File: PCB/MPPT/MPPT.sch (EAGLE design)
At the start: 2 parts, among them IC1 ACS711KEXLT-15AB-T, IC2 ACS711KEXLT-15AB-T

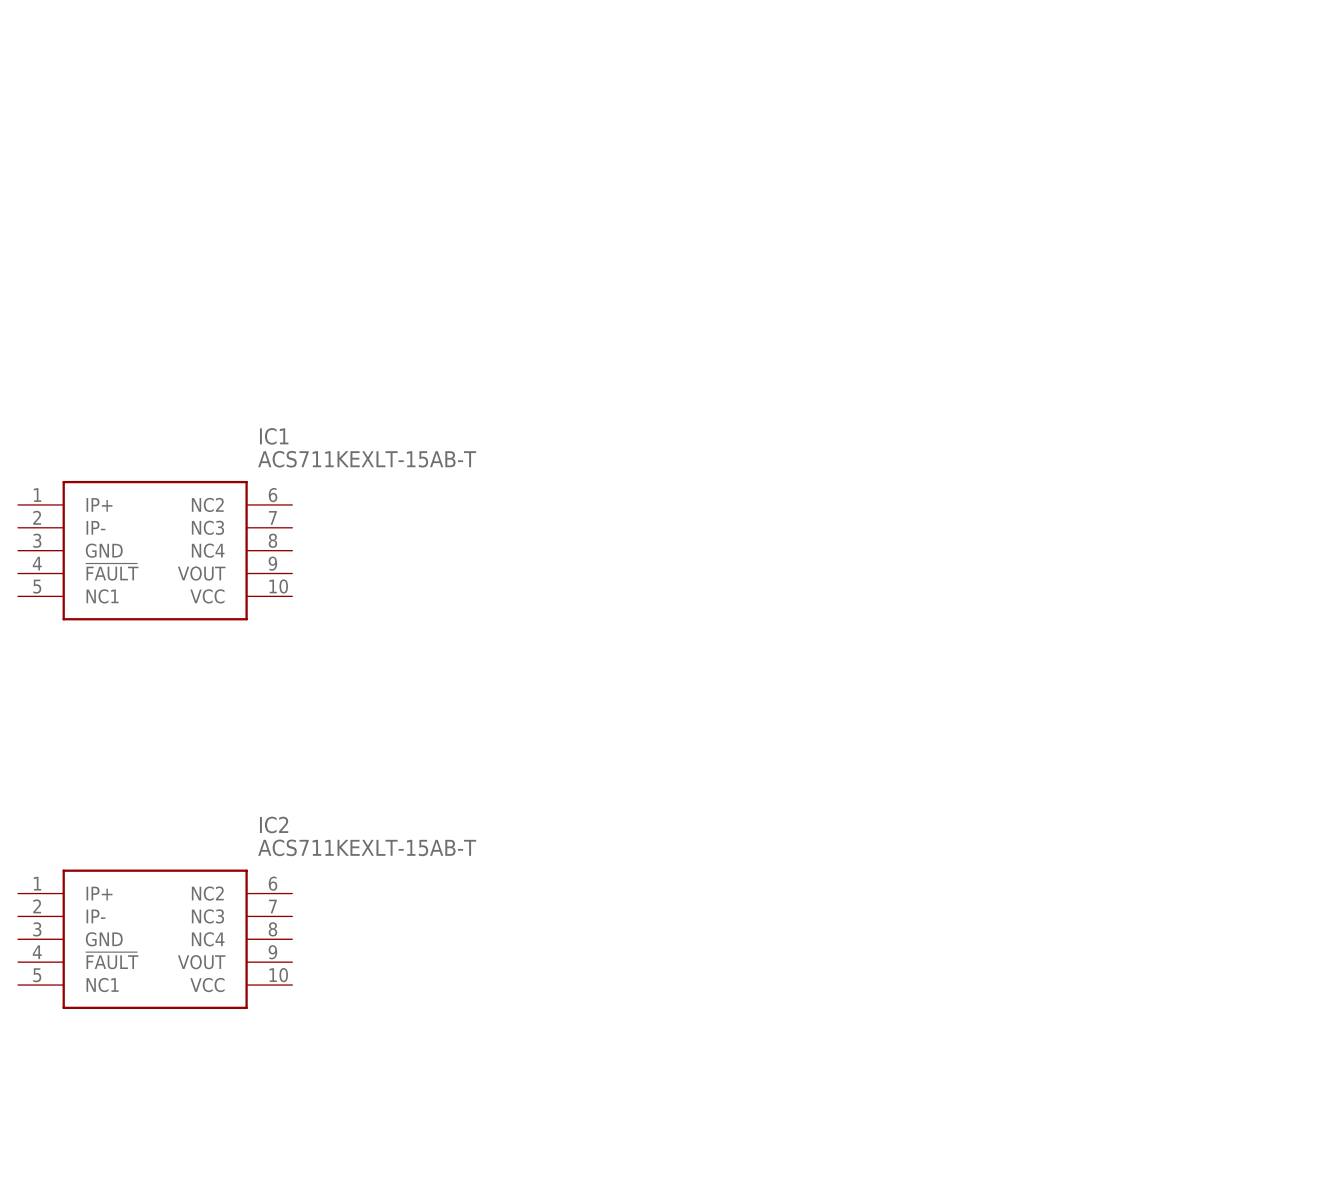
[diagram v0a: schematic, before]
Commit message: nothing
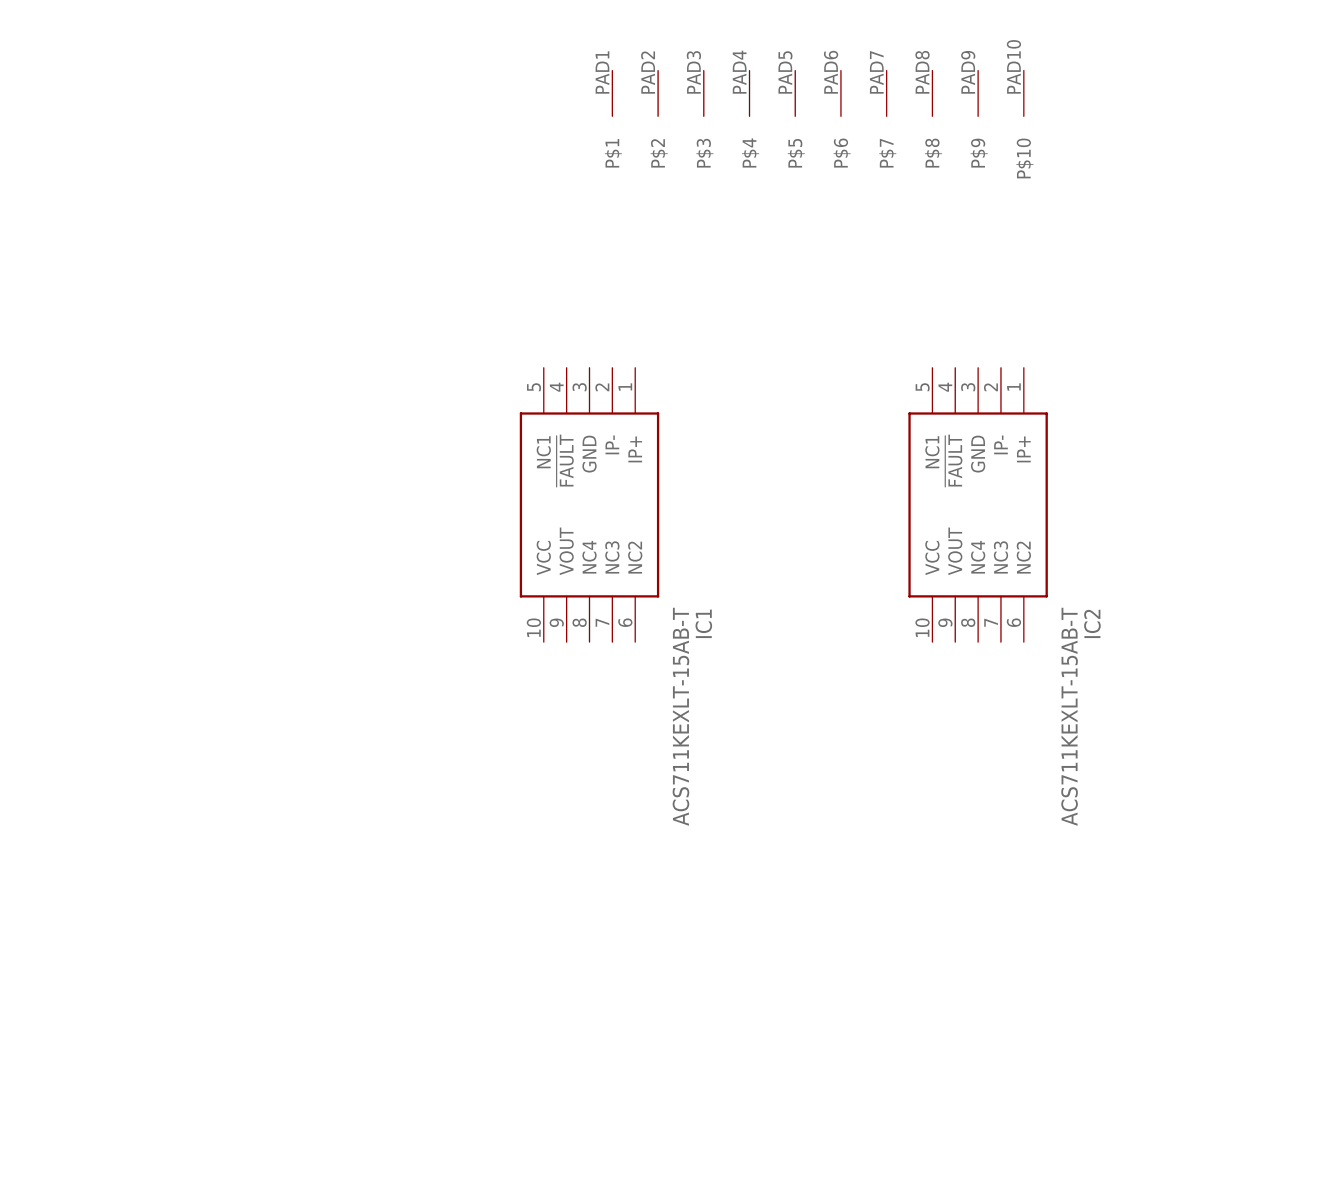
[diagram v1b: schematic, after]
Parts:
- added U$1: CONN-KF2EDG-10(5.08)E-BAYPLUGGABLECONNECTORS, Stuff_I_Use:CONN-KF2EDG-10(5.08)E-BAYPLUGGABLECONNECTORS
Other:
- moved on the sheet: IC1, IC2
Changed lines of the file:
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@@
 <part name="IC1" library="SamacSys_Parts" deviceset="ACS711KEXLT-15AB-T" device=""/>
 <part name="IC2" library="SamacSys_Parts" deviceset="ACS711KEXLT-15AB-T" device=""/>
+<part name="U$1" library="Stuff_I_Use" deviceset="CONN-KF2EDG-10(5.08)" device="E-BAYPLUGGABLECONNECTORS"/>
 </parts>
 <sheets>
@@
 </plain>
 <instances>
-<instance part="IC1" gate="G$1" x="35.56" y="142.24"/>
-<instance part="IC2" gate="G$1" x="35.56" y="99.06"/>
+<instance part="IC1" gate="G$1" x="104.14" y="157.48" rot="R270"/>
+<instance part="IC2" gate="G$1" x="147.32" y="157.48" rot="R270"/>
+<instance part="U$1" gate="G$1" x="121.92" y="185.42"/>
 </instances>
 <busses>

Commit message: Start of Board Design
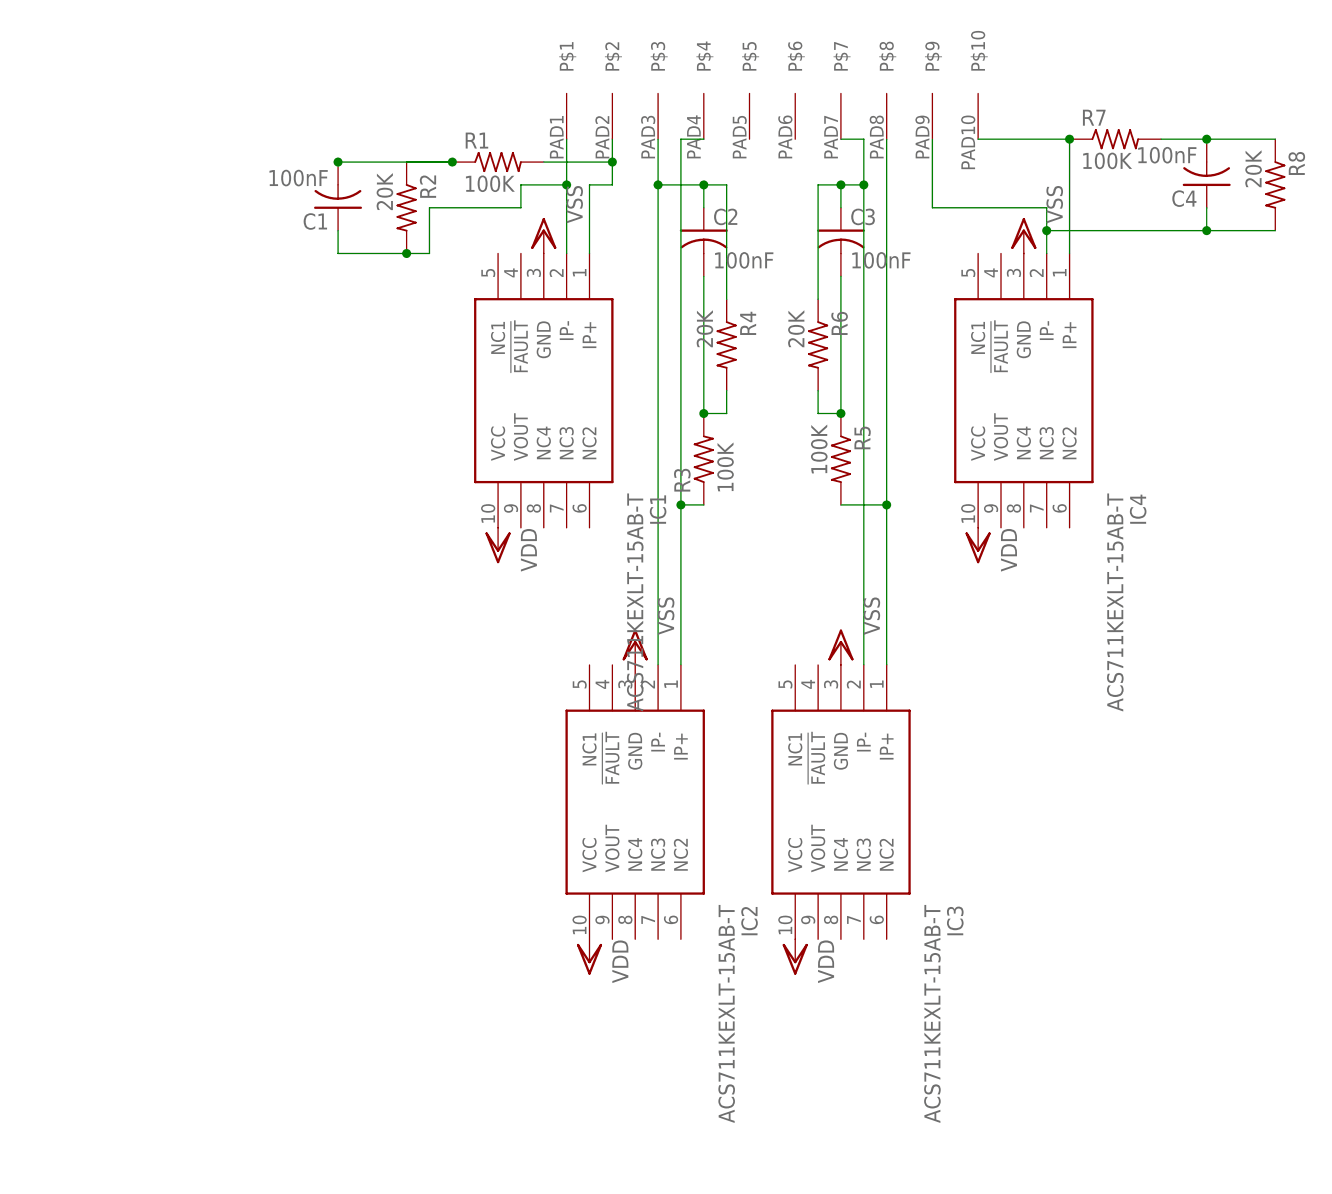
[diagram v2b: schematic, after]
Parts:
- added C1, C2, C3, C4: 100nF, resistor:C-USC0603
- added IC3, IC4: ACS711KEXLT-15AB-T, SamacSys_Parts:ACS711KEXLT-15AB-T
- added R1, R3, R5, R7: 100K, resistor:R-US_R0603
- added R2, R4, R6, R8: 20K, resistor:R-US_R0603
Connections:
- new net N$1: C1.2, R1.1, R2.1
- new net N$2: C2.1, IC2.IP-, R4.1, U$1.P$3
- new net N$3: IC2.IP+, R3.1, U$1.P$4
- new net N$4: C2.2, R3.2, R4.2
- new net N$5: C3.2, R5.1, R6.2
- new net N$6: C4.2, R7.2, R8.1
- new net N$7: IC4.IP+, R7.1, U$1.P$10
- new net N$8: C4.1, IC4.IP-, R8.2, U$1.P$9
- new net N$B_1+: IC3.IP+, R5.2, U$1.P$8
- new net N$B_1-: C3.1, IC3.IP-, R6.1, U$1.P$7
- new net N$PV_1+: IC1.IP+, R1.2, U$1.P$2
- new net N$PV_1-: C1.1, IC1.IP-, R2.2, U$1.P$1
- new net VDD: IC1.VCC, IC2.VCC, IC3.VCC, IC4.VCC
- new net VSS: IC1.GND, IC2.GND, IC3.GND, IC4.GND
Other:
- moved on the sheet: IC1, IC2

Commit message: progress
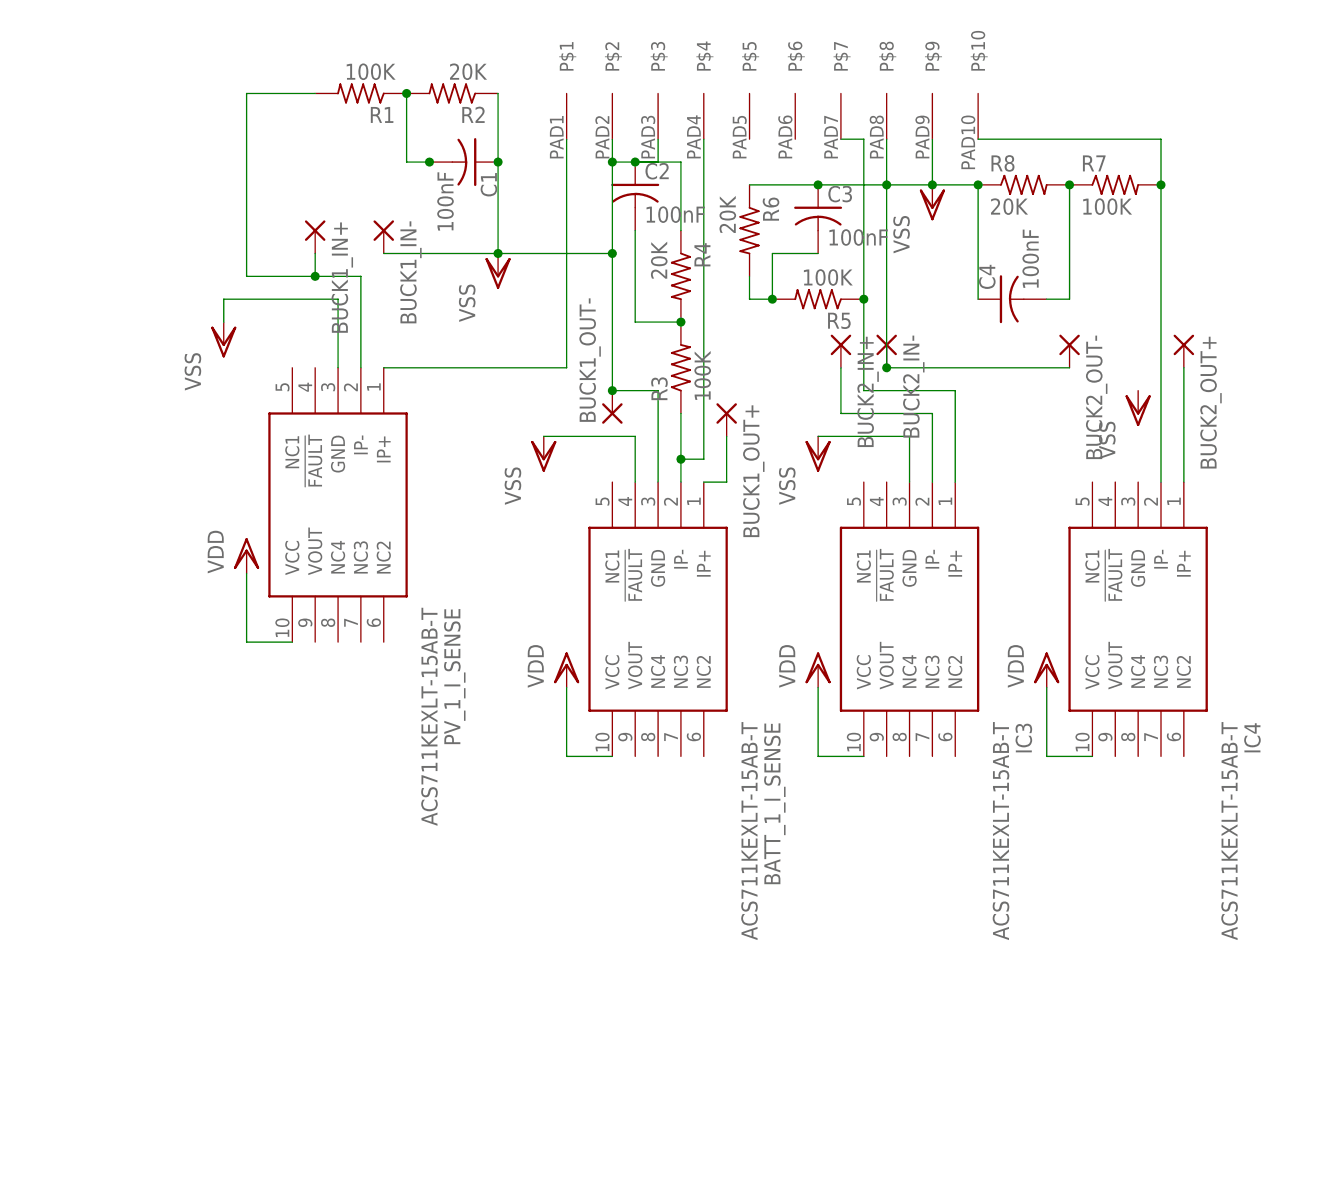
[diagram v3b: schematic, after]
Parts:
- removed IC1, IC2: ACS711KEXLT-15AB-T, SamacSys_Parts:ACS711KEXLT-15AB-T
- added BATT_1_I_SENSE, PV_1_I_SENSE: ACS711KEXLT-15AB-T, SamacSys_Parts:ACS711KEXLT-15AB-T
- added BUCK1_IN+, BUCK1_IN-, BUCK1_OUT+, BUCK1_OUT-, BUCK2_IN+, BUCK2_IN-, BUCK2_OUT+, BUCK2_OUT-: (no value), wirepad:3,81/1,4
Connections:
- removed net N$5 (its old number): C3.2, R5.1, R6.2
- removed net N$B_1+: IC3.IP+, R5.2, U$1.P$8
- removed net N$B_1-: C3.1, IC3.IP-, R6.1, U$1.P$7
- removed net N$PV_1+: IC1.IP+, R1.2, U$1.P$2
- removed net N$PV_1-: C1.1, IC1.IP-, R2.2, U$1.P$1
- new net N$10: C3.2, R5.2, R6.2
- new net N$11: IC4.IP-, R7.2, U$1.P$10
- new net N$12: C4.2, R7.1, R8.2
- new net N$4: BATT_1_I_SENSE.IP+, BUCK1_OUT+.P
- new net N$9: BUCK2_IN+.P, IC3.IP-
- net N$1: now also PV_1_I_SENSE.IP+, U$1.P$1; no longer C1.2, R1.1, R2.1
- net N$2: now also BUCK1_IN+.P, PV_1_I_SENSE.IP-, R1.2; no longer C2.1, IC2.IP-, R4.1, U$1.P$3
- net N$3: now also C1.2, R1.1, R2.2; no longer IC2.IP+, R3.1, U$1.P$4
- net N$6: now also BATT_1_I_SENSE.IP-, R3.1, U$1.P$4; no longer C4.2, R7.2, R8.1
- net N$7: now also BUCK2_OUT+.P; no longer R7.1, U$1.P$10
- net N$8: now also IC3.IP+, R5.1, U$1.P$7; no longer C4.1, IC4.IP-, R8.2, U$1.P$9
- net VDD: now also BATT_1_I_SENSE.VCC, PV_1_I_SENSE.VCC; no longer IC1.VCC, IC2.VCC
- net VSS: now also BATT_1_I_SENSE.!FAULT, BATT_1_I_SENSE.GND, BUCK1_IN-.P, BUCK1_OUT-.P, BUCK2_IN-.P, BUCK2_OUT-.P, C1.1, C2.1, C3.1, C4.1, PV_1_I_SENSE.GND, R2.1, R4.1, R6.1, R8.1, U$1.P$2, U$1.P$3, U$1.P$8, U$1.P$9; no longer IC1.GND, IC2.GND, IC4.GND
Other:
- moved on the sheet: C1, C2, C3, C4, IC3, IC4, R1, R2, R3, R4, R5, R6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
